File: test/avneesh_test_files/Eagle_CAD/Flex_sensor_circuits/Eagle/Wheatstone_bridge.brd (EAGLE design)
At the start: 160 x 100 mm, 20 parts

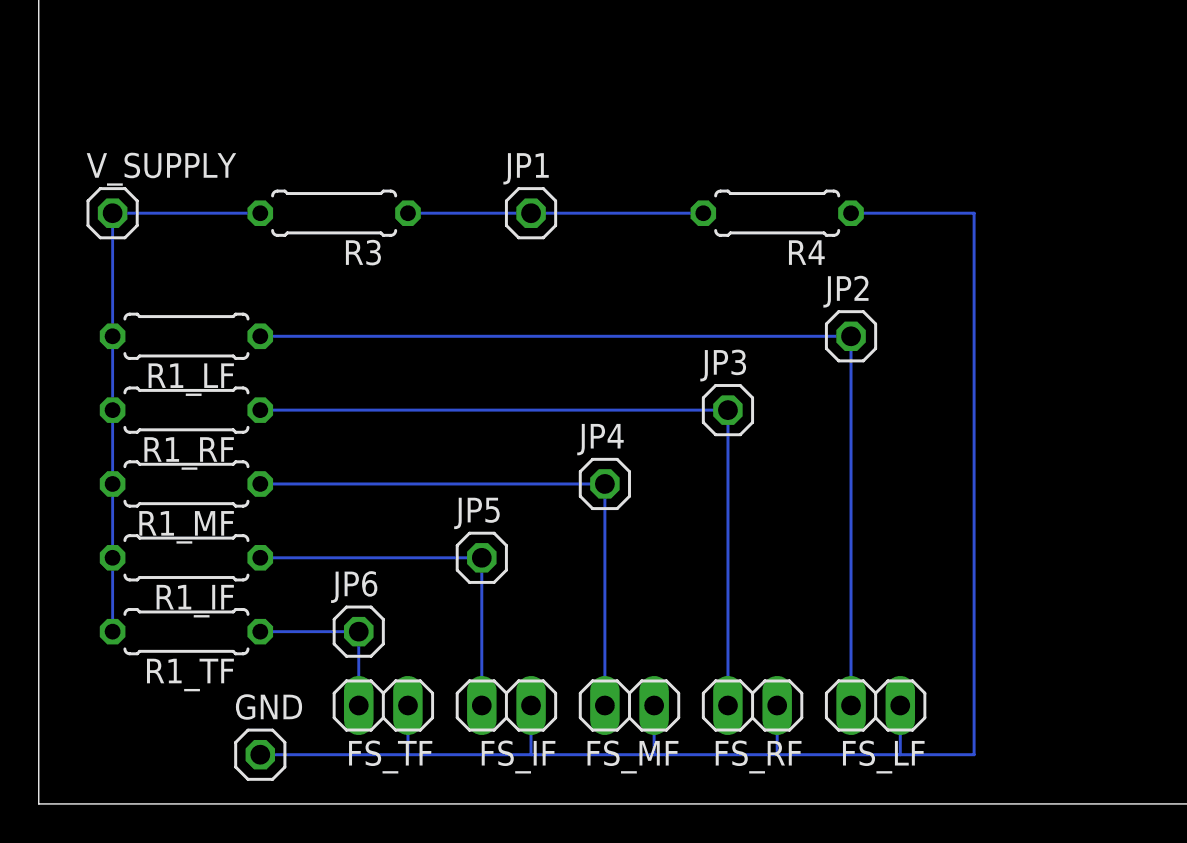
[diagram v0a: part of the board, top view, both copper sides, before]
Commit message: Made changes to the CAD files
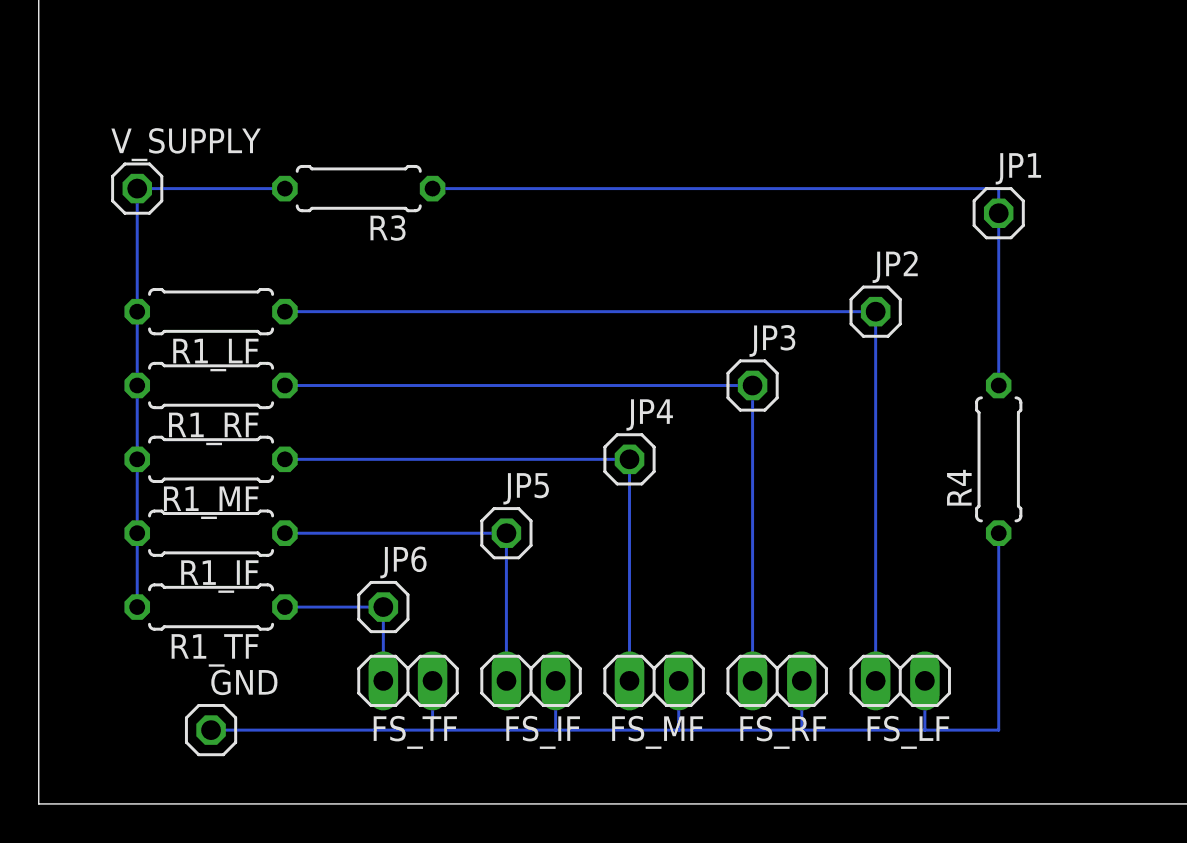
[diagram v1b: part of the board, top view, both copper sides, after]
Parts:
- moved JP1 24.1 mm to (49.5, 30.5)
- moved R4 17.1 mm to (49.5, 17.8), turned to 90 degrees
- moved GND 2.84 mm to (8.89, 3.81)
- moved FS_LF 1.80 mm to (44.5, 6.35)
- moved FS_RF 1.80 mm to (38.1, 6.35)
- moved JP2 1.80 mm to (43.2, 25.4)
- moved R1_IF 1.80 mm to (8.89, 14.0)
- moved JP5 1.80 mm to (24.1, 14.0)
- moved R3 1.80 mm to (16.5, 31.8)
- moved R1_LF 1.80 mm to (8.89, 25.4)
- moved R1_MF 1.80 mm to (8.89, 17.8)
- moved R1_RF 1.80 mm to (8.89, 21.6)
- moved R1_TF 1.80 mm to (8.89, 10.2)
- moved V_SUPPLY 1.80 mm to (5.08, 31.8)
- moved FS_IF 1.80 mm to (25.4, 6.35)
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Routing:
- net N$2: track 15.2 -> 39.4 mm
- net GND: track 83.8 -> 63.5 mm
